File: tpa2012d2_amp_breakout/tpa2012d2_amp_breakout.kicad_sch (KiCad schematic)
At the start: 7 parts, among them J101 Conn_01x07_Female, J102 SPK L, J103 SPK R, J104 AudioJack3, J105 SD, J106 G0, J107 G1

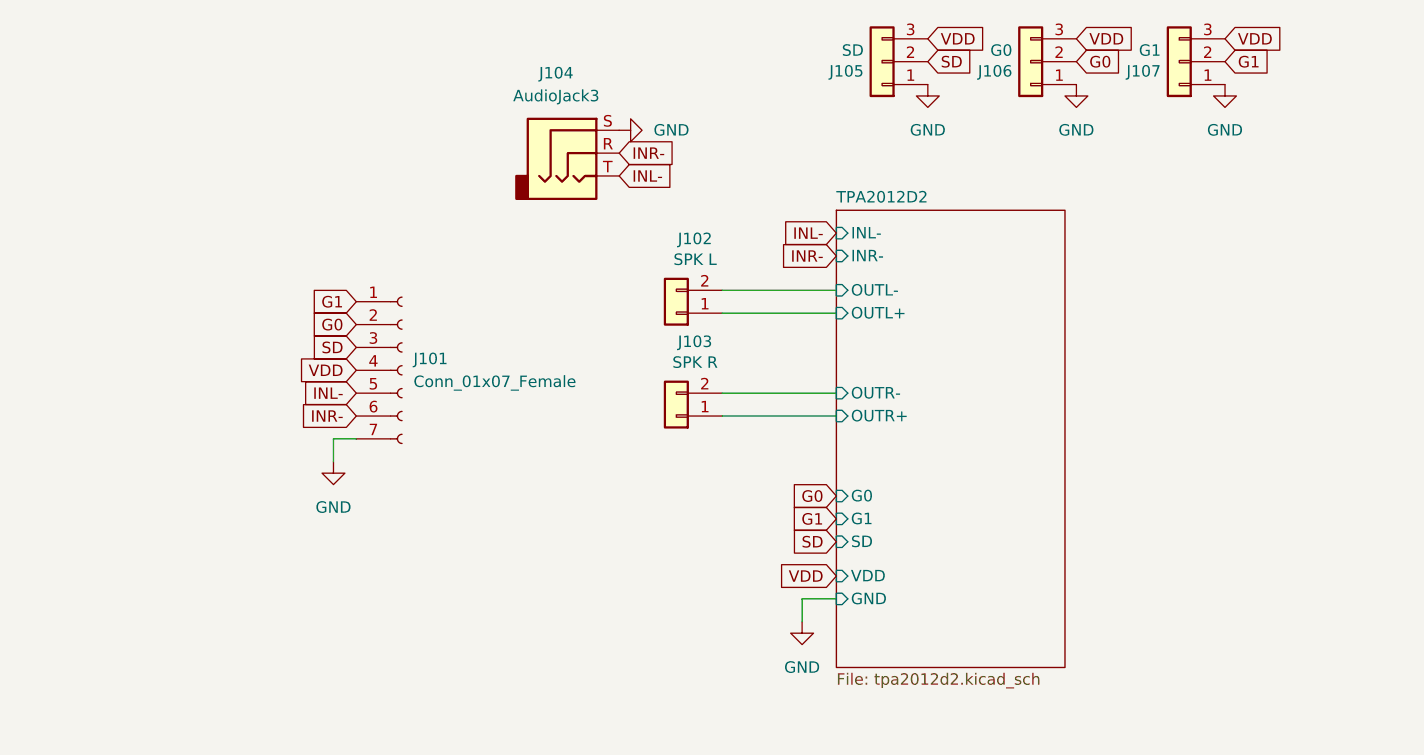
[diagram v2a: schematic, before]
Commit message: final touches + v1 jlcpcb fab files
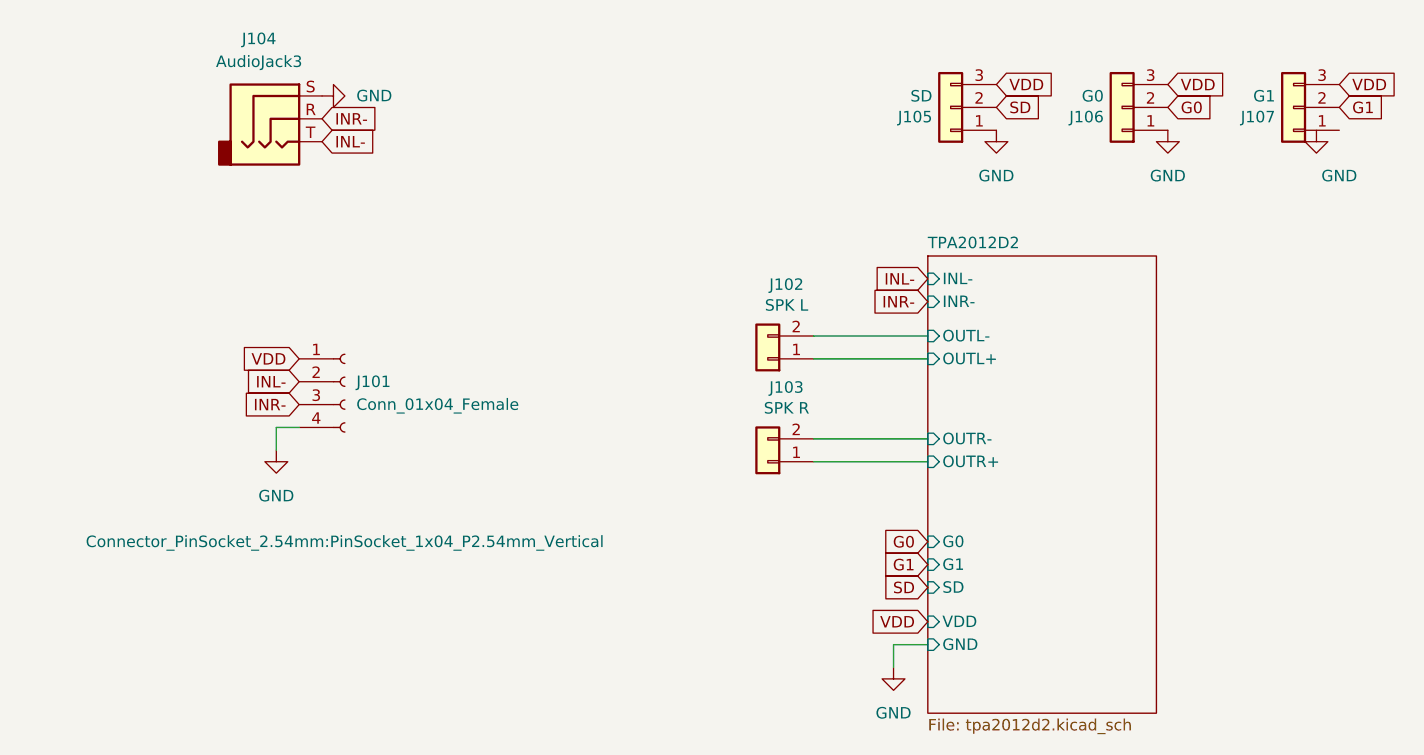
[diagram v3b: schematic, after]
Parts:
- removed J101: Conn_01x07_Female, Connector_PinSocket_2.54mm:PinSocket_1x07_P2.54mm_Vertical, symbol Connector:Conn_01x07_Female
- added J101: Conn_01x04_Female, Connector_PinSocket_2.54mm:PinSocket_1x04_P2.54mm_Vertical, symbol Connector:Conn_01x04_Female
- J104: LCSC Part (none) -> C707224; MSCS Part C707224 -> (none)
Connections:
- net GND: now also J101.4 (Pin_4); no longer J107.1 (Pin_1)
- net INL-: now also J101.2 (Pin_2)
- net INR-: now also J101.3 (Pin_3)
- net VDD: now also J101.1 (Pin_1)
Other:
- moved on the sheet: J102, J103, J104, J105, J106, J107
